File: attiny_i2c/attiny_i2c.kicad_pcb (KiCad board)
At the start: 2 copper layers, 12 parts, among them IC1 ATTINY25-S, P1 CONN_02X03, P2 CONN_01X06

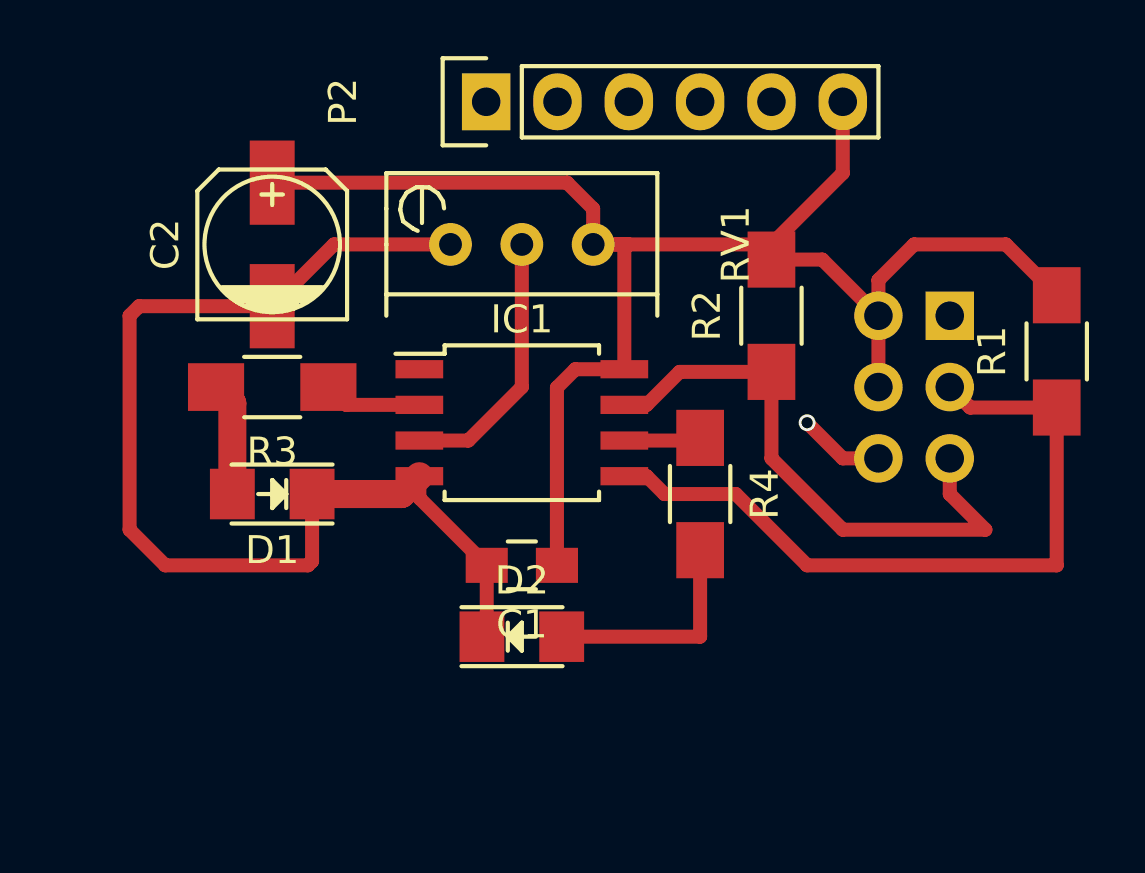
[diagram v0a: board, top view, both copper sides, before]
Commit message: More or less current schematics
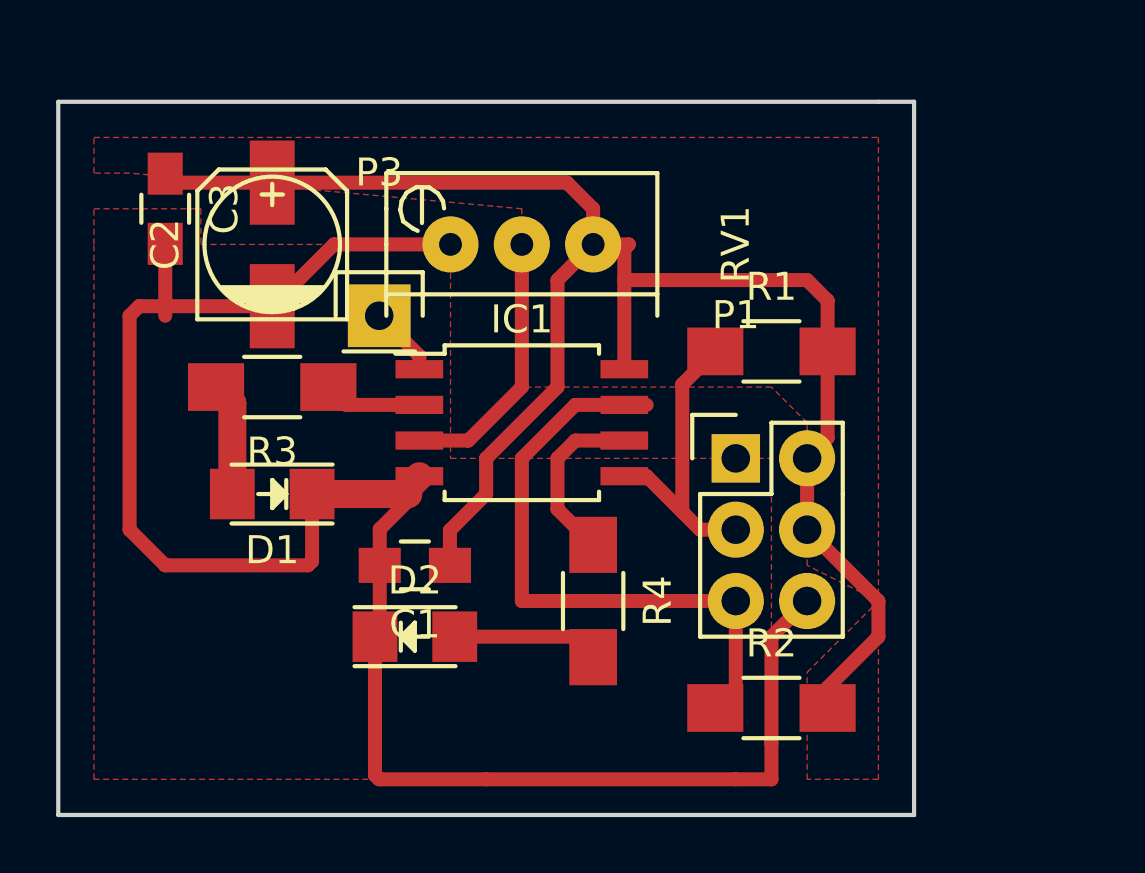
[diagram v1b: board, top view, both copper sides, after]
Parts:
- removed P2: CONN_01X06, Pin_Headers:Pin_Header_Straight_1x06
- added C3: C_Small, Capacitors_SMD:C_0805_HandSoldering, F.Cu at (102.9, 33.0)
- added P3: CONN_01X01, Pin_Headers:Pin_Header_Straight_1x01, F.Cu at (110.5, 36.8)
- P1: moved to F.Cu
- moved R2 14.0 mm to (124.5, 50.8), turned to 0 degrees
- moved R1 10.2 mm to (124.5, 38.1), turned to 0 degrees
- moved P1 9.16 mm to (123.2, 41.9), turned to 0 degrees
- moved R4 5.39 mm to (118.1, 47.0)
- moved C1 3.81 mm to (111.8, 45.7)
- moved D2 3.81 mm to (111.8, 48.3)
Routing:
- net GND: track 43.5 -> 68.3 mm, vias 1 -> 0
- net I2C_SDA: track 26.4 -> 11.0 mm
- net LED2: track 2.74 -> 6.25 mm
- net +5V: track 57.2 -> 60.5 mm
- net Net-(D2-Pad2): track 8.01 -> 5.23 mm
- net PRG_RST: track 0.00 -> 2.50 mm
- net I2C_SCL: track 20.5 -> 22.0 mm
- added copper zone on F.Cu, net +5V
- added copper zone on F.Cu, net GND
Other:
- board outline added: 30.5 x 25.4 mm
